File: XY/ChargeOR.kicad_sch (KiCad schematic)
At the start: 8 parts, among them U13 LTC4376CDHD_PBF, U9 SI3865DDV-T1-GE3

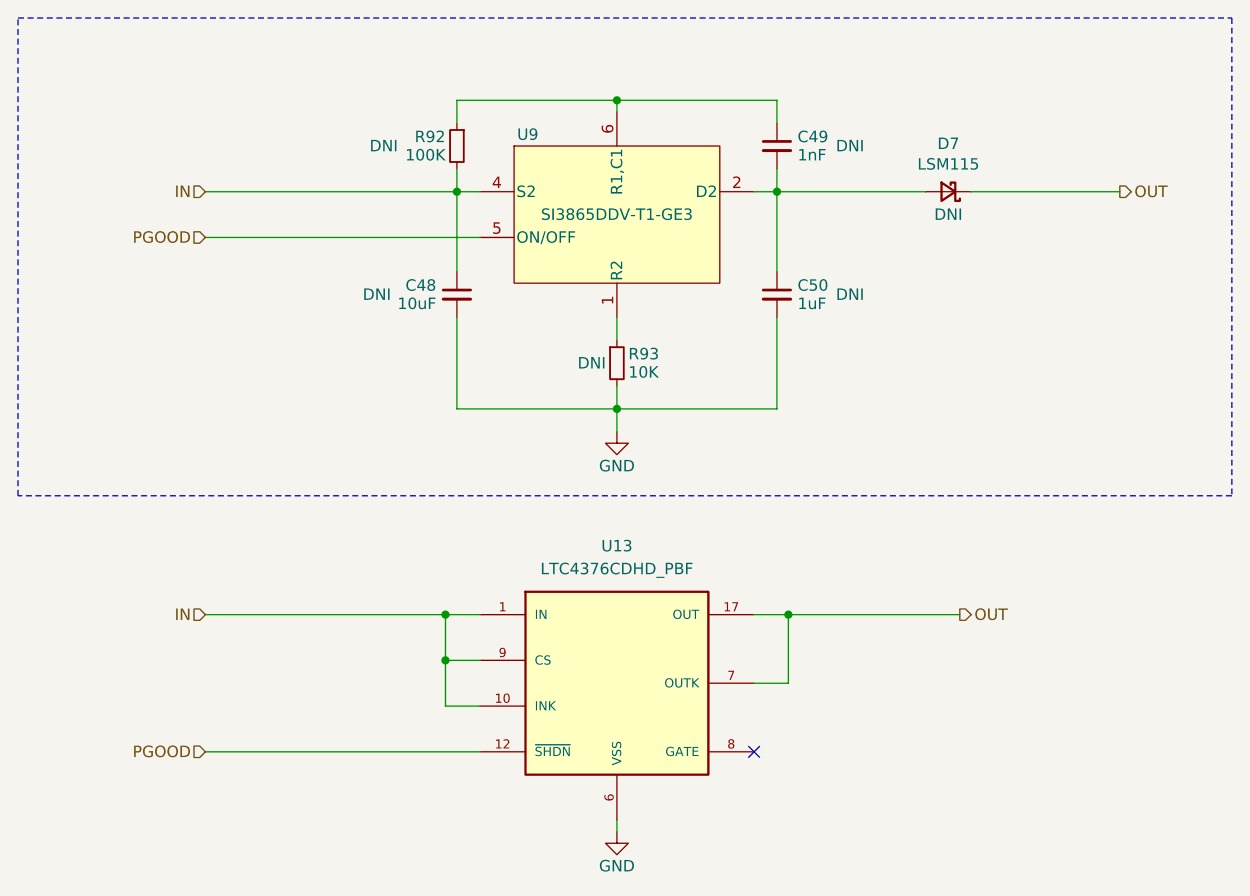
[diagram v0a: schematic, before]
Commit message: MPPT fixes
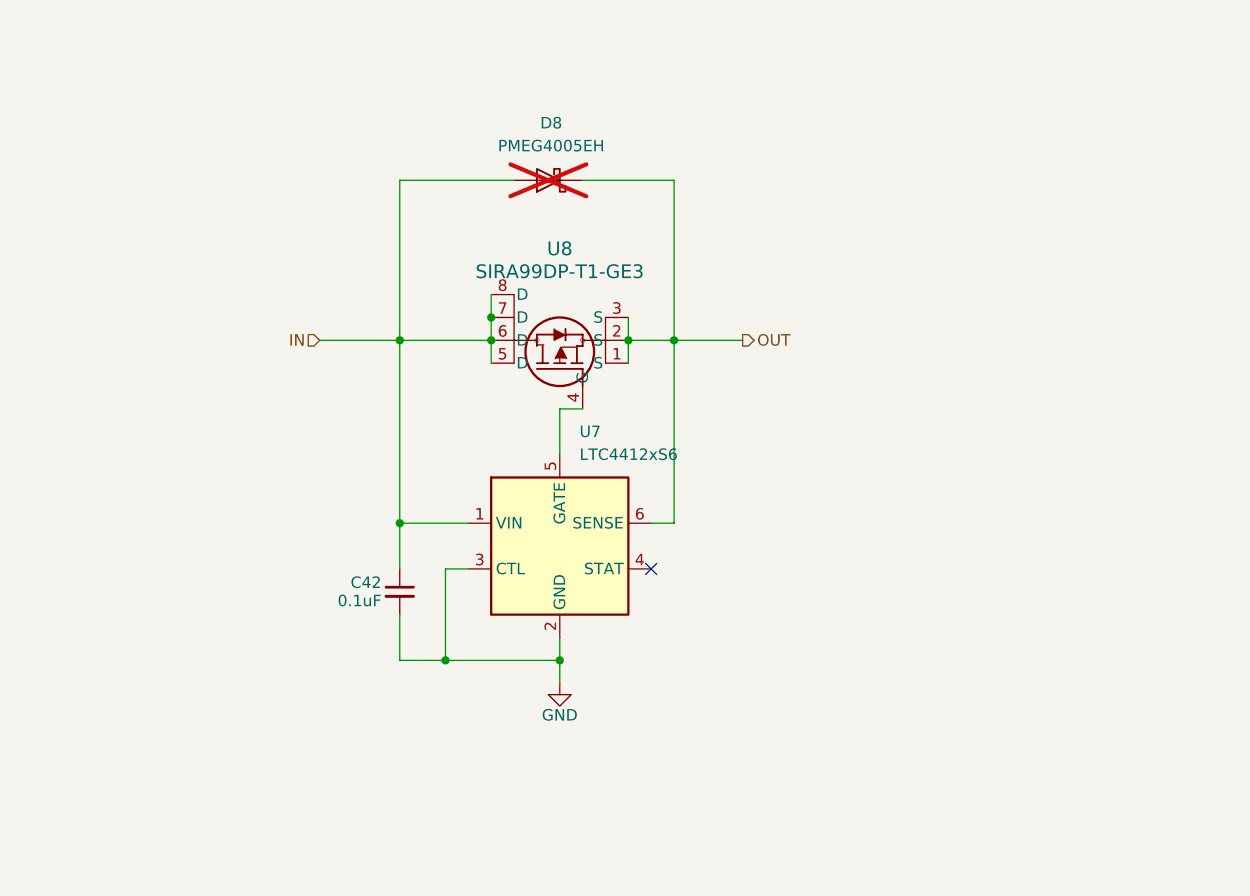
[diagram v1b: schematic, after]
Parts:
- removed C48: 10uF, Capacitor_SMD:C_1206_3216Metric, symbol Device:C_Small
- removed C49: 1nF, Capacitor_SMD:C_0603_1608Metric, symbol Device:C_Small
- removed C50: 1uF, Capacitor_SMD:C_1206_3216Metric, symbol Device:C_Small
- removed D7: LSM115, SolarPanels:DO-214BA_MCH, symbol Device:D_Schottky_Small
- removed R92: 100K, Resistor_SMD:R_0603_1608Metric, symbol Device:R_Small
- removed R93: 10K, Resistor_SMD:R_0603_1608Metric, symbol Device:R_Small
- removed U13: LTC4376CDHD_PBF, Package_DFN_QFN:DFN-16-1EP_4x5mm_P0.5mm_EP2.44x4.34mm, symbol SolarPanels:LTC4376CDHD_PBF
- removed U9: SI3865DDV-T1-GE3, Package_TO_SOT_SMD:SOT-23-6, symbol SolarPanels:SI3865DDV-T1-GE3
- added C42: 0.1uF, Capacitor_SMD:C_0603_1608Metric, symbol Device:C_Small
- added D8: PMEG4005EH, Diode_SMD:D_SOD-123F, symbol Diode:PMEG4005EH
- added U7: LTC4412xS6, Package_TO_SOT_SMD:TSOT-23-6, symbol Power_Management:LTC4412xS6
- added U8: SIRA99DP-T1-GE3, SolarPanels:MOSFET_7DP-T1-GE3_VIS, symbol Argus-Misc:SIRA99DP-T1-GE3
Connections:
- net GND: now also C42.2, U7.2 (GND), U7.3 (CTL)
- net IN: now also C42.1, D8.2 (A), U7.1 (VIN), U8.5 (D), U8.6 (D), U8.7 (D), U8.8 (D)
- net OUT: now also D8.1 (K), U7.6 (SENSE), U8.1 (S), U8.2 (S), U8.3 (S)
- new net: U7.5 (GATE), U8.4 (G)
